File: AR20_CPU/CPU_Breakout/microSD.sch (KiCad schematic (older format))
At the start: 6 parts, among them U2 MCP1700_SOT23

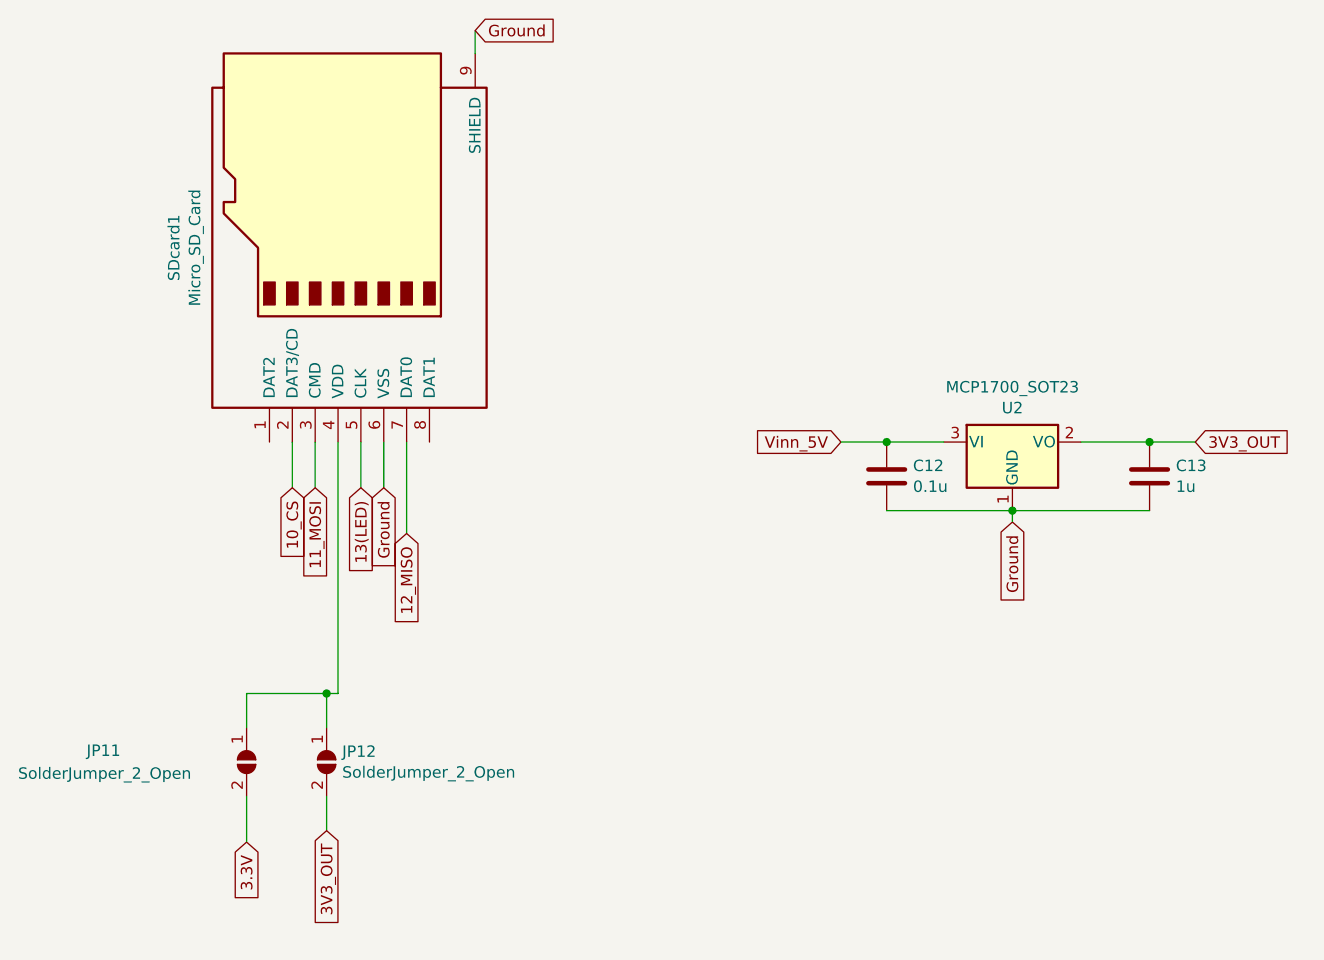
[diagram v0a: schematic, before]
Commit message: E2
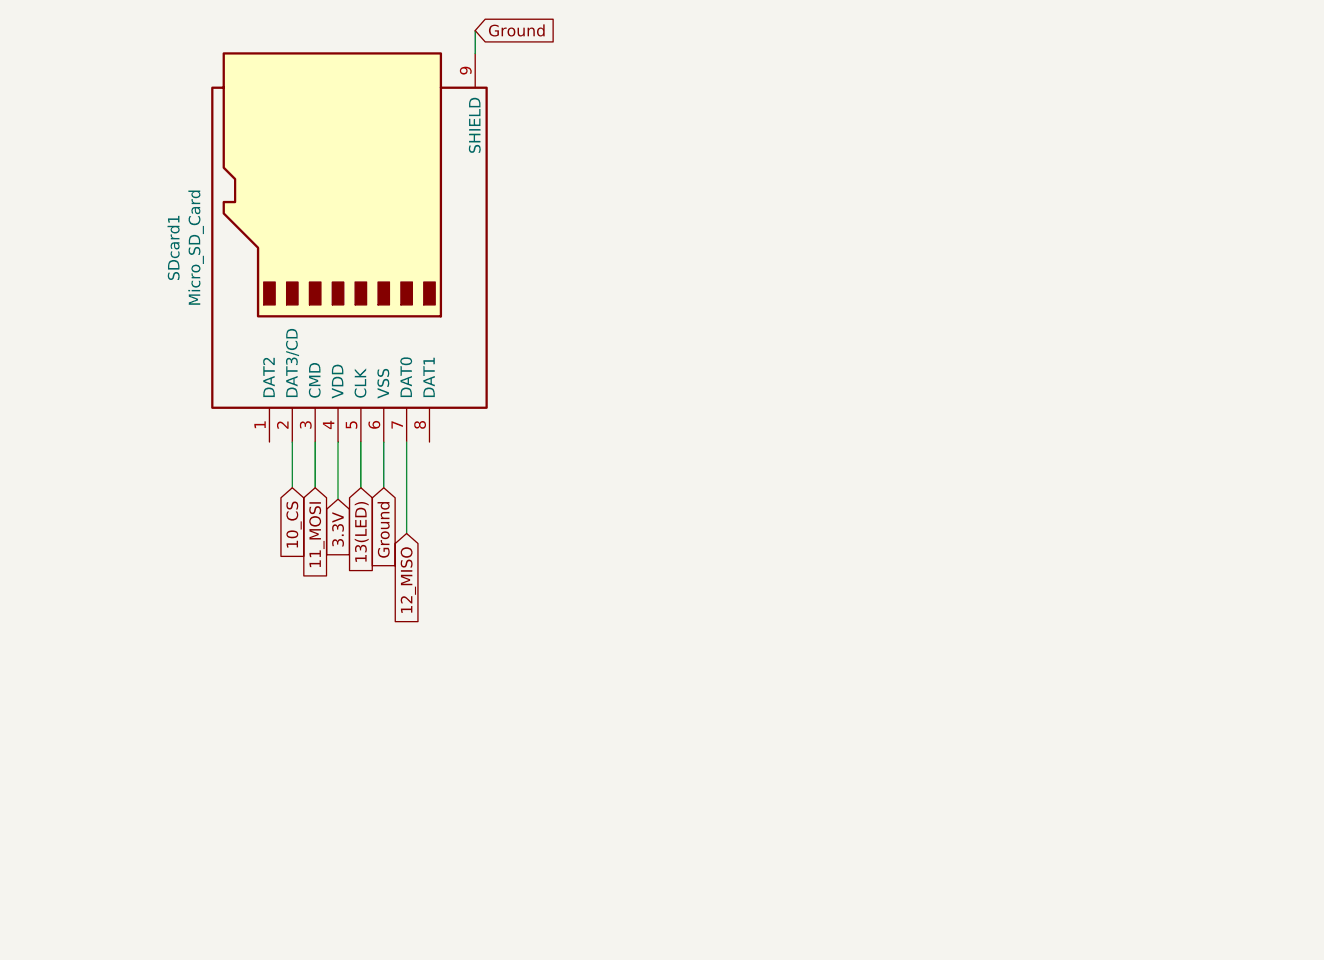
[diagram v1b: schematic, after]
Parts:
- removed C12: 0.1u, Capacitor_SMD:C_0603_1608Metric, symbol Device:C
- removed C13: 1u, Capacitor_SMD:C_0603_1608Metric, symbol Device:C
- removed JP11, JP12: SolderJumper_2_Open, Jumper:SolderJumper-2_P1.3mm_Open_RoundedPad1.0x1.5mm, symbol Jumper:SolderJumper_2_Open
- removed U2: MCP1700_SOT23, Package_TO_SOT_SMD:SOT-23, symbol Regulator_Linear:MCP1700-3302E_SOT23
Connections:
- net 3.3V: now also SDcard1.4 (VDD)
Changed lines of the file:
@@
 $EndDescr
-Wire Wire Line
-	8300 3800 8300 3850
-Text GLabel 8300 3850 3    50   Input ~ 0
-Ground
-Text GLabel 7550 3500 0    50   Input ~ 0
-Vinn_5V
-$Comp
-L Regulator_Linear:MCP1700-3302E_SOT23 U?
-U 1 1 5DFCE3D9
-P 8300 3500
-AR Path="/5DFCE3D9" Ref="U?"  Part="1"
-AR Path="/5DFCB53C/5DFCE3D9" Ref="U2"  Part="1"
-AR Path="/5DE8C4DF/5DFCE3D9" Ref="U2"  Part="1"
-F 0 "U2" H 8300 3649 50  0000 C CNN
-F 1 "MCP1700_SOT23" H 8300 3740 50  0000 C CNN
-F 2 "Package_TO_SOT_SMD:SOT-23" H 8300 3725 50  0001 C CNN
-F 3 "http://ww1.microchip.com/downloads/en/DeviceDoc/20001826D.pdf" H 8300 3500 50  0001 C CNN
-	1    8300 3500
-	1    0    0    -1
-$EndComp
 Wire Wire Line
 	5950 1800 5950 1700
@@
 Text GLabel 5950 1700 2    50   Input ~ 0
 Ground
-Wire Wire Line
-	7750 3800 8300 3800
-Connection ~ 8300 3800
-Wire Wire Line
-	8300 3800 8900 3800
-Wire Wire Line
-	7550 3500 7750 3500
-Wire Wire Line
-	8000 3500 7750 3500
-Connection ~ 7750 3500
-$Comp
-L Device:C C12
-U 1 1 5DE5A450
-P 7750 3650
-F 0 "C12" H 7635 3604 50  0000 R CNN
-F 1 "0.1u" H 7635 3695 50  0000 R CNN
-F 2 "Capacitor_SMD:C_0603_1608Metric" H 7788 3500 50  0001 C CNN
-F 3 "~" H 7750 3650 50  0001 C CNN
-	1    7750 3650
-	-1   0    0    1
-$EndComp
-Text GLabel 9100 3500 2    50   Input ~ 0
-3V3_OUT
-Wire Wire Line
-	8900 3500 8600 3500
-Wire Wire Line
-	9100 3500 8900 3500
-Connection ~ 8900 3500
-$Comp
-L Device:C C13
-U 1 1 5DE59DD0
-P 8900 3650
-F 0 "C13" H 8785 3604 50  0000 R CNN
-F 1 "1u" H 8785 3695 50  0000 R CNN
-F 2 "Capacitor_SMD:C_0603_1608Metric" H 8938 3500 50  0001 C CNN
-F 3 "~" H 8900 3650 50  0001 C CNN
-	1    8900 3650
-	-1   0    0    1
-$EndComp
 Text GLabel 5150 3700 3    50   Input ~ 0
 10_CS
@@
 Text GLabel 5250 3700 3    50   Input ~ 0
 11_MOSI
-Text GLabel 5300 5200 3    50   Input ~ 0
-3V3_OUT
 Wire Wire Line
 	5650 3500 5650 3900
@@
 Wire Wire Line
 	5150 3500 5150 3700
-$Comp
-L Jumper:SolderJumper_2_Open JP12
-U 1 1 5DEFC778
-P 5300 4900
-F 0 "JP12" V 5254 4968 50  0000 L CNN
-F 1 "SolderJumper_2_Open" V 5345 4968 50  0000 L CNN
-F 2 "Jumper:SolderJumper-2_P1.3mm_Open_RoundedPad1.0x1.5mm" H 5300 4900 50  0001 C CNN
-F 3 "~" H 5300 4900 50  0001 C CNN
-	1    5300 4900
-	0    1    1    0
-$EndComp
-$Comp
-L Jumper:SolderJumper_2_Open JP11
-U 1 1 5DF02FDA
-P 4950 4900
-F 0 "JP11" V 4900 4200 50  0000 L CNN
-F 1 "SolderJumper_2_Open" V 5000 3900 50  0000 L CNN
-F 2 "Jumper:SolderJumper-2_P1.3mm_Open_RoundedPad1.0x1.5mm" H 4950 4900 50  0001 C CNN
-F 3 "~" H 4950 4900 50  0001 C CNN
-	1    4950 4900
-	0    1    1    0
-$EndComp
-Wire Wire Line
-	5300 5200 5300 5050
-Wire Wire Line
-	5300 4750 5300 4600
-Wire Wire Line
-	4950 4750 4950 4600
-Wire Wire Line
-	5350 4600 5300 4600
-Wire Wire Line
-	5350 3500 5350 4600
-Wire Wire Line
-	5300 4600 4950 4600
-Connection ~ 5300 4600
-Text GLabel 4950 5250 3    50   Input ~ 0
+Text GLabel 5350 3750 3    50   Input ~ 0
 3.3V
 Wire Wire Line
-	4950 5050 4950 5250
+	5350 3500 5350 3750
 $EndSCHEMATC
